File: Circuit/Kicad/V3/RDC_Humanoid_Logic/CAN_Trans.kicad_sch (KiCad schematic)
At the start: 18 parts, among them U1 ISOW1044

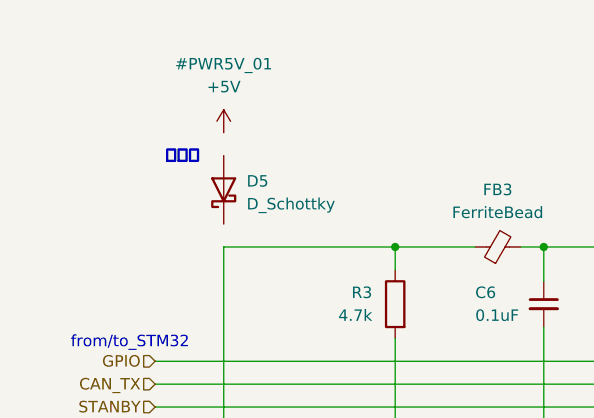
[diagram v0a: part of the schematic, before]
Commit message: 修正箇所を修正した
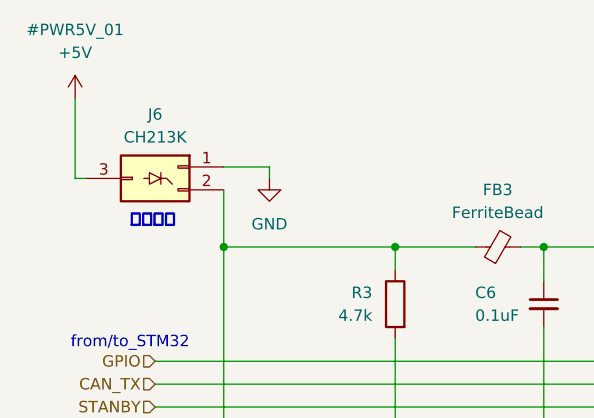
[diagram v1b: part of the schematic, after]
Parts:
- removed D5: D_Schottky, symbol Device:D_Schottky
- added J6: CH213K, Package_TO_SOT_SMD:SOT-23-3, symbol Connector_Generic:Conn_02x02_Counter_Clockwise
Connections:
- net +5V: now also J6.3 (Pin_3)
- net GND: now also J6.1 (Pin_1)
- net at FB2.1, FB3.1, R3.1: now also J6.2 (Pin_2)
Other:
- note added: "修正済み"
- note removed: "要修正"
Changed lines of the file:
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@@
 	(generator_version "9.0")
 	(paper "A4")
-	(text "要修正"
+	(text "修正済み"
 		(exclude_from_sim no)
-		(at 86.868 58.674 0)
+		(at 83.566 65.786 0)
 		(effects
 			(font
@@
 				(thickness 0.254)
 				(bold yes)
-				(color 99 0 0 1)
+				(color 0 99 0 1)
 			)
 		)
@@
 	)
 	(junction
+		(at 91.44 68.58)
+		(diameter 0)
+		(color 0 0 0 0)
+	)
+	(junction
 		(at 177.8 69.85)
 		(diameter 0)
@@
 	(wire
 		(pts
+			(xy 96.52 59.69) (xy 96.52 60.96)
+		)
+		(stroke
+			(width 0)
+			(type default)
+		)
+	)
+	(wire
+		(pts
 			(xy 162.56 114.3) (xy 173.99 114.3)
 		)
@@
 	(wire
 		(pts
+			(xy 91.44 68.58) (xy 110.49 68.58)
+		)
+		(stroke
+			(width 0)
+			(type default)
+		)
+	)
+	(wire
+		(pts
 			(xy 83.82 88.9) (xy 139.7 88.9)
 		)
@@
 	(wire
 		(pts
-			(xy 91.44 68.58) (xy 110.49 68.58)
-		)
-		(stroke
-			(width 0)
-			(type default)
-		)
-	)
-	(wire
-		(pts
 			(xy 201.93 99.06) (xy 205.74 99.06)
 		)
@@
 	(wire
 		(pts
+			(xy 76.2 60.96) (xy 74.93 60.96)
+		)
+		(stroke
+			(width 0)
+			(type default)
+		)
+	)
+	(wire
+		(pts
 			(xy 163.83 78.74) (xy 163.83 69.85)
 		)
@@
 	(wire
 		(pts
+			(xy 91.44 59.69) (xy 96.52 59.69)
+		)
+		(stroke
+			(width 0)
+			(type default)
+		)
+	)
+	(wire
+		(pts
 			(xy 160.02 88.9) (xy 170.18 88.9)
 		)
@@
 	(wire
 		(pts
+			(xy 91.44 62.23) (xy 91.44 68.58)
+		)
+		(stroke
+			(width 0)
+			(type default)
+		)
+	)
+	(wire
+		(pts
 			(xy 190.5 104.14) (xy 190.5 99.06)
 		)
@@
 		(pts
 			(xy 171.45 96.52) (xy 171.45 99.06)
+		)
+		(stroke
+			(width 0)
+			(type default)
+		)
+	)
+	(wire
+		(pts
+			(xy 74.93 60.96) (xy 74.93 52.07)
 		)
 		(stroke
@@
 				(path "/2bec3ac6-4176-417a-a2e5-e81844f01e63/4e0cc178-8164-45af-8b1c-3daea8e76e2d"
 					(reference "C13")
-					(unit 1)
-				)
-			)
-		)
-	)
-	(symbol
-		(lib_id "Device:D_Schottky")
-		(at 91.44 62.23 90)
-		(unit 1)
-		(exclude_from_sim no)
-		(in_bom yes)
-		(on_board yes)
-		(dnp no)
-		(fields_autoplaced yes)
-		(property "Reference" "D5"
-			(at 93.98 61.2774 90)
-			(effects
-				(font
-					(size 1.27 1.27)
-				)
-				(justify right)
-			)
-		)
-		(property "Value" "D_Schottky"
-			(at 93.98 63.8174 90)
-			(effects
-				(font
-					(size 1.27 1.27)
-				)
-				(justify right)
-			)
-		)
-		(property "Footprint" ""
-			(at 91.44 62.23 0)
-			(effects
-				(font
-					(size 1.27 1.27)
-				)
-				(hide yes)
-			)
-		)
-		(property "Datasheet" "~"
-			(at 91.44 62.23 0)
-			(effects
-				(font
-					(size 1.27 1.27)
-				)
-				(hide yes)
-			)
-		)
-		(property "Description" "Schottky diode"
-			(at 91.44 62.23 0)
-			(effects
-				(font
-					(size 1.27 1.27)
-				)
-				(hide yes)
-			)
-		)
-		(pin "2"
-		)
-		(pin "1"
-		)
-		(instances
-			(project ""
-				(path "/2bec3ac6-4176-417a-a2e5-e81844f01e63/2ffb334c-541d-4787-8f08-8f2b280267fd"
-					(reference "D5")
-					(unit 1)
-				)
-				(path "/2bec3ac6-4176-417a-a2e5-e81844f01e63/4e0cc178-8164-45af-8b1c-3daea8e76e2d"
-					(reference "D6")
 					(unit 1)
 				)
@@
 	(symbol
 		(lib_id "power:+5V")
-		(at 91.44 55.88 0)
+		(at 74.93 52.07 0)
 		(unit 1)
 		(exclude_from_sim no)
@@
 		(dnp no)
 		(property "Reference" "#PWR5V_01"
-			(at 91.44 48.26 0)
+			(at 74.93 44.45 0)
 			(effects
 				(font
@@
 		)
 		(property "Value" "+5V"
-			(at 91.44 50.8 0)
+			(at 74.93 46.99 0)
 			(effects
 				(font
@@
 		)
 		(property "Footprint" ""
-			(at 91.44 55.88 0)
+			(at 74.93 52.07 0)
 			(effects
 				(font
@@
 		)
 		(property "Datasheet" ""
-			(at 91.44 55.88 0)
+			(at 74.93 52.07 0)
 			(effects
 				(font
@@
 		)
 		(property "Description" ""
-			(at 91.44 55.88 0)
+			(at 74.93 52.07 0)
 			(effects
 				(font
@@
 					(unit 1)
 				)
+			)
+		)
+	)
+	(symbol
+		(lib_id "Connector_Generic:Conn_02x02_Counter_Clockwise")
+		(at 86.36 59.69 0)
+		(mirror y)
+		(unit 1)
+		(exclude_from_sim no)
+		(in_bom yes)
+		(on_board yes)
+		(dnp no)
+		(property "Reference" "J6"
+			(at 83.82 53.848 0)
+			(effects
+				(font
+					(size 1.27 1.27)
+				)
+			)
+		)
+		(property "Value" "CH213K"
+			(at 83.82 56.388 0)
+			(effects
+				(font
+					(size 1.27 1.27)
+				)
+			)
+		)
+		(property "Footprint" "Package_TO_SOT_SMD:SOT-23-3"
+			(at 86.36 59.69 0)
+			(effects
+				(font
+					(size 1.27 1.27)
+				)
+				(hide yes)
+			)
+		)
+		(property "Datasheet" "https://akizukidenshi.com/goodsaffix/CH213.pdf"
+			(at 86.36 59.69 0)
+			(effects
+				(font
+					(size 1.27 1.27)
+				)
+				(hide yes)
+			)
+		)
+		(property "Description" "Generic connector, double row, 02x02, counter clockwise pin numbering scheme (similar to DIP package numbering), script generated (kicad-library-utils/schlib/autogen/connector/)"
+			(at 86.106 66.548 0)
+			(effects
+				(font
+					(size 1.27 1.27)
+				)
+				(hide yes)
+			)
+		)
+		(pin "1"
+		)
+		(pin "2"
+		)
+		(pin "3"
+		)
+		(instances
+			(project ""
+				(path "/2bec3ac6-4176-417a-a2e5-e81844f01e63/2ffb334c-541d-4787-8f08-8f2b280267fd"
+					(reference "J6")
+					(unit 1)
+				)
+				(path "/2bec3ac6-4176-417a-a2e5-e81844f01e63/4e0cc178-8164-45af-8b1c-3daea8e76e2d"
+					(reference "J7")
+					(unit 1)
+				)
+			)
+		)
+	)
+	(symbol
+		(lib_id "power:GND")
+		(at 96.52 60.96 0)
+		(unit 1)
+		(exclude_from_sim no)
+		(in_bom yes)
+		(on_board yes)
+		(dnp no)
+		(fields_autoplaced yes)
+		(property "Reference" "#PWR012"
+			(at 96.52 67.31 0)
+			(effects
+				(font
+					(size 1.27 1.27)
+				)
+				(hide yes)
+			)
+		)
+		(property "Value" "GND"
+			(at 96.52 66.04 0)
+			(effects
+				(font
+					(size 1.27 1.27)
+				)
+			)
+		)
+		(property "Footprint" ""
+			(at 96.52 60.96 0)
+			(effects
+				(font
+					(size 1.27 1.27)
+				)
+				(hide yes)
+			)
+		)
+		(property "Datasheet" ""
+			(at 96.52 60.96 0)
+			(effects
+				(font
+					(size 1.27 1.27)
+				)
+				(hide yes)
+			)
+		)
+		(property "Description" ""
+			(at 96.52 60.96 0)
+			(effects
+				(font
+					(size 1.27 1.27)
+				)
+			)
+		)
+		(pin "1"
+		)
+		(instances
+			(project "RDC_Humanoid_Logic"
+				(path "/2bec3ac6-4176-417a-a2e5-e81844f01e63/2ffb334c-541d-4787-8f08-8f2b280267fd"
+					(reference "#PWR012")
+					(unit 1)
+				)
+				(path "/2bec3ac6-4176-417a-a2e5-e81844f01e63/4e0cc178-8164-45af-8b1c-3daea8e76e2d"
+					(reference "#PWR016")
+					(unit 1)
+				)
